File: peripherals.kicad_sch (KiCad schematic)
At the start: 23 parts, among them CN1 PJ-3059-B, CN2 PJ-3059-B, SW3 K2-1808SN-A4SW, SW4 K2-1808SN-A4SW, U48 2.54-1*4, U49 2.54-1*4, U50 LMV358IDR

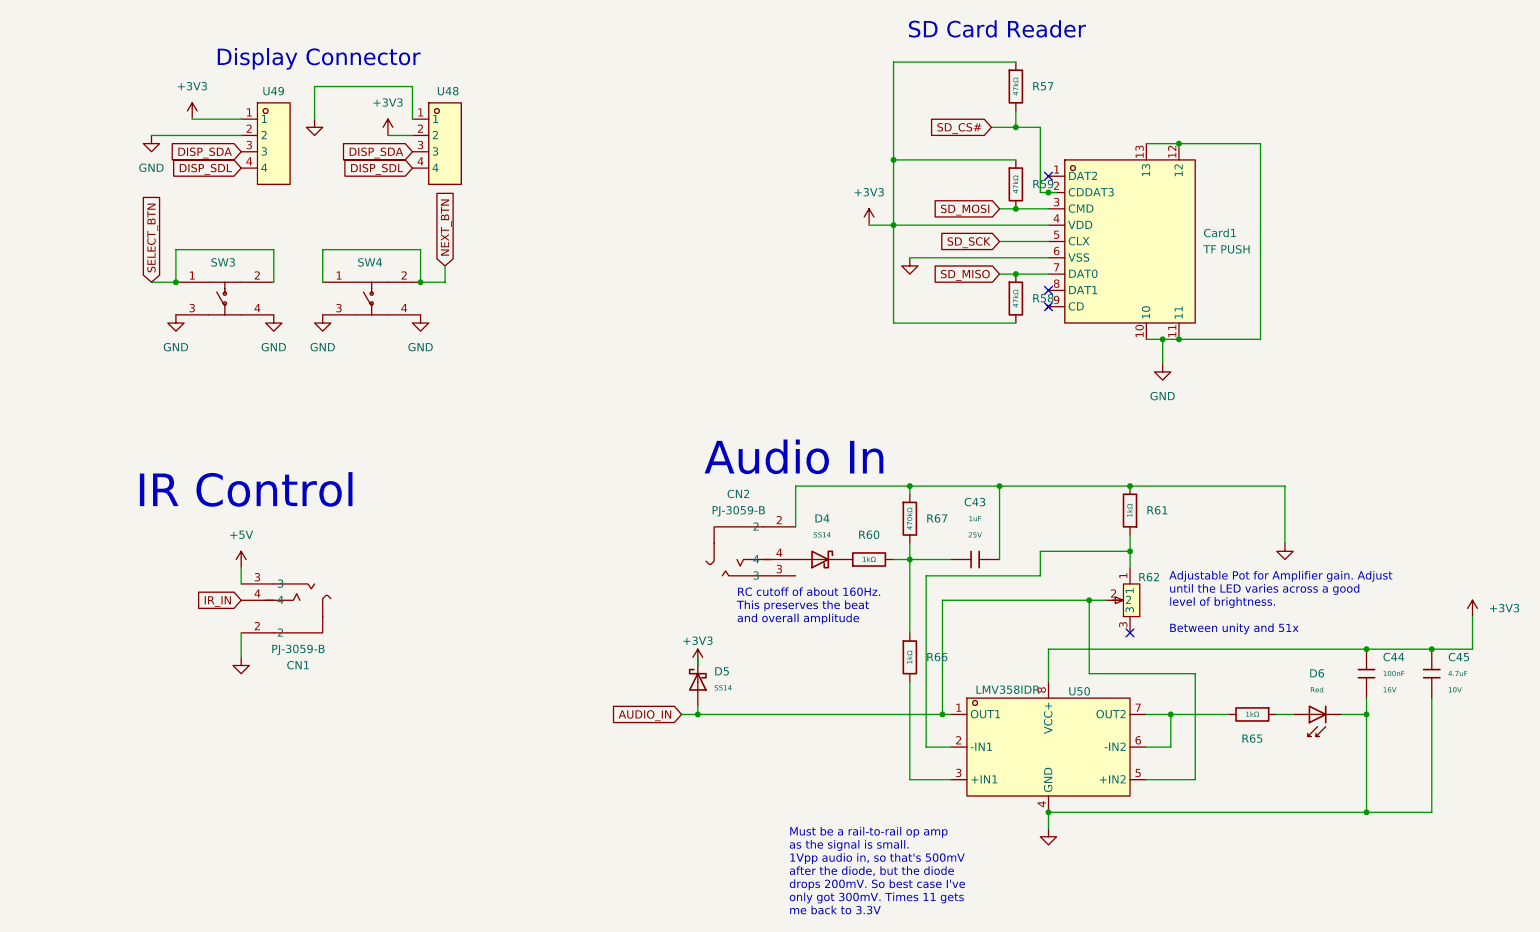
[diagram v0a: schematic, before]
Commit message: Working on errata
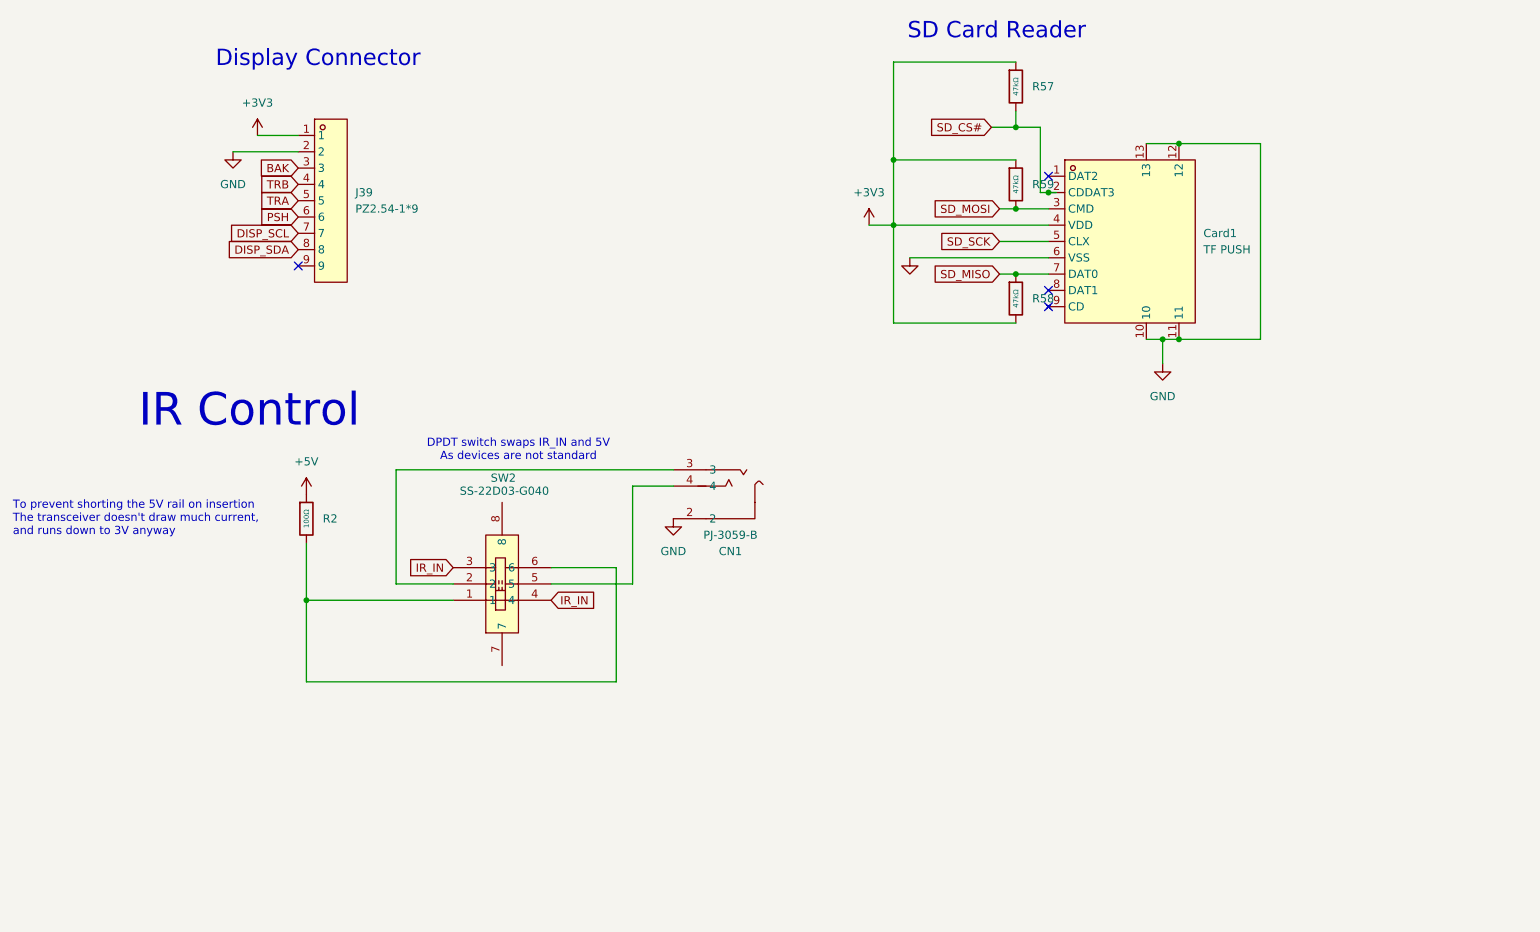
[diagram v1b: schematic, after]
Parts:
- removed C43: 1uF, PixelBlit:C_0402, symbol PixelBlit:0402,1uF
- removed C44: 100nF, PixelBlit:C_0402, symbol PixelBlit:0402,100nF
- removed C45: 4.7uF, PixelBlit:C_0402, symbol PixelBlit:0402,4.7uF
- removed CN2: PJ-3059-B, PixelBlit:AUDIO-TH_XKB_PJ-3059-B, symbol PixelBlit:PJ-3059-B
- removed D4, D5: SS14, PixelBlit:D_SMA, symbol PixelBlit:Schottky,SS14
- removed D6: Red, PixelBlit:D_0603, symbol PixelBlit:LED,0603,Red
- removed R60, R61: 1kΩ, PixelBlit:R_0603, symbol PixelBlit:0603,1kΩ
- removed R62: 3362P-1-503LF, PixelBlit:RES-ADJ-TH_3362P, symbol PixelBlit:3362P-1-503LF
- removed R65: 1kΩ, PixelBlit:R_0402, symbol PixelBlit:0402,1kΩ
- removed R66: 1kΩ, PixelBlit:R_0402, symbol PixelBlit:0402,1kΩ_1
- removed R67: 470kΩ, PixelBlit:R_0402, symbol PixelBlit:0402,470kΩ
- removed SW3, SW4: K2-1808SN-A4SW, PixelBlit:KEY-SMD_4P-L4.2-W3.2-P2.20-LS5.1-TL, symbol PixelBlit:K2-1808SN-A4SW
- removed U48, U49: 2.54-1*4, PixelBlit:HDR-TH_4P-P2.54-V-M-1, symbol PixelBlit:2.54-1*4
- removed U50: LMV358IDR, PixelBlit:SOIC-8_L4.9-W3.9-P1.27-LS6.0-BL, symbol PixelBlit:LMV358IDR
- added J39: PZ2.54-1*9, EasyEDA:HDR-TH_9P-P2.54-V-M, symbol EasyEDA:PZ2.54-1*9
- added R2: 100Ω, PCM_JLCPCB:R_0603, symbol PCM_JLCPCB-Resistors:0603,100Ω
- added SW2: SS-22D03-G040, EasyEDA:SW-TH_SS-22D03-G4, symbol EasyEDA:SS-22D03-G040
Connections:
- net +3V3: now also J39.1
- net +5V: now also R2.1; no longer CN1.3
- net DISP_SDA: now also J39.8
- net GND: now also J39.2
- net IR_IN: now also SW2.3, SW2.4; no longer CN1.4
- new net: R2.2, SW2.1, SW2.6
- new net: CN1.3, SW2.2
- new net: CN1.4, SW2.5
- new net BAK: J39.3
- new net DISP_SCL: J39.7
- new net PSH: J39.6
- new net TRA: J39.5
- new net TRB: J39.4
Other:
- note added: "DPDT switch swaps IR_IN and 5V As devices are not standard"
- note added: "To prevent shorting the 5V rail on insertion The transceiver doesn't draw much current, and runs down to 3V anyway"
- note removed: "Adjustable Pot for Amplifier gain. Adjust until the LED varies across a good level of brightness. Between unity and 51x"
- note removed: "Audio In"
- note removed: "Must be a rail-to-rail op amp as the signal is small. 1Vpp audio in, so that's 500mV after the diode, but the diode drops 200mV. So best case I've only got 300mV. Times 11 gets me back to 3.3V"
- note removed: "RC cutoff of about 160Hz. This preserves the beat and overall amplitude"
- moved on the sheet: CN1
